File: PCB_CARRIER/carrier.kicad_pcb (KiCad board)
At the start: 6 copper layers, 69.6 x 46 mm, 87 parts, among them J1 SODIMM-260_Split, J2 Micro_SD_Card_Det2, Q1 BSS138, Q2 BSS138, Q3 BSS138, Q4 BC817-40, SW1 SW_DIP_x04, U1 SN74LVC8T245, U2 SN74LVC8T245, U3 SN74LVC8T245, U4 RT9742GGJ5

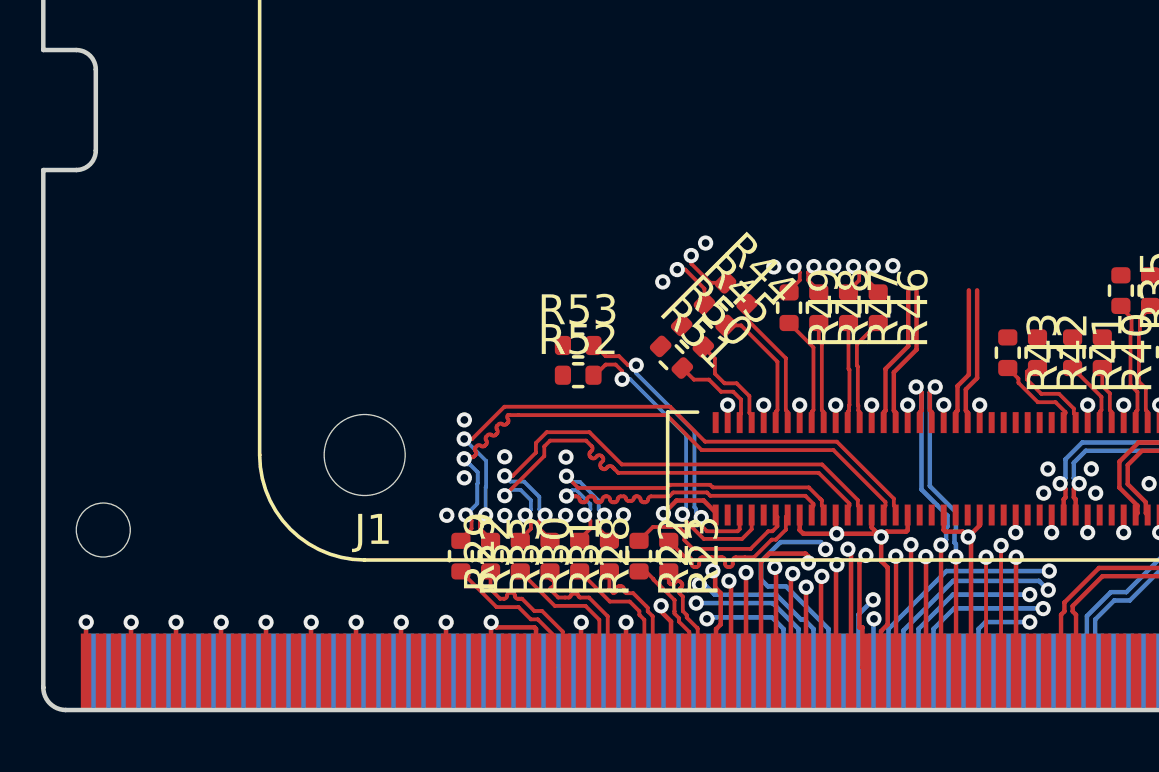
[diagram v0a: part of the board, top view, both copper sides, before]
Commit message: yes I'm still routing CSI
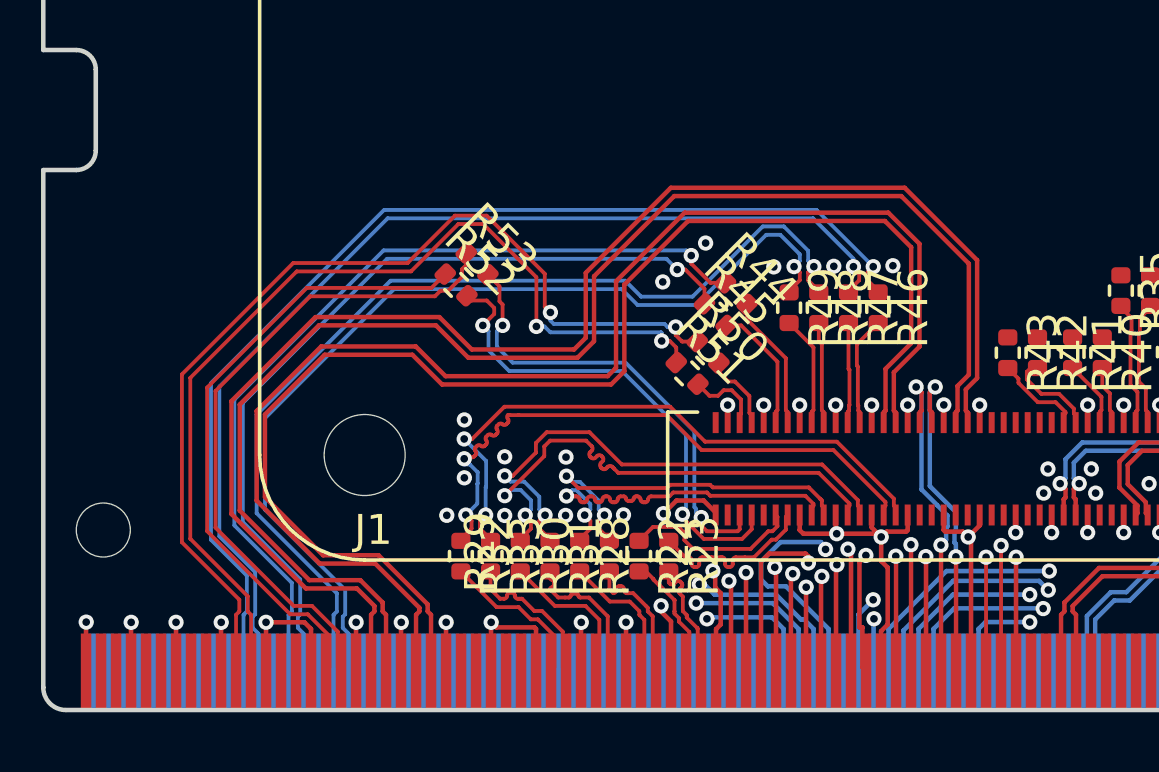
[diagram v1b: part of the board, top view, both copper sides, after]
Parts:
- moved R52 5.06 mm to (113.8, 85.8), turned to -45 degrees
- moved R53 4.33 mm to (114.5, 85.1), turned to -45 degrees
- moved R50 0.75 mm to (122.2, 88.1)
- moved R51 0.75 mm to (121.5, 88.8)
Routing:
- net USB3-1-RX_N: track 4.59 -> 48.6 mm
- net USB3-1-RX_P: track 4.59 -> 47.7 mm
- net USB3-1-TX_N: track 4.73 -> 46.2 mm
- net USB3-1-TX_P: track 4.73 -> 45.2 mm
- net dCSI-1_D0_N: track 1.08 -> 36.5 mm
- net dCSI-1_D0_P: track 1.08 -> 35.5 mm
- net dCSI-1_D2_N: track 0.00 -> 32.8 mm, vias 0 -> 2
- net dCSI-1_D2_P: track 0.00 -> 32.3 mm, vias 0 -> 2
- net dCSI-1_D1_N: track 1.09 -> 33.2 mm
- net dCSI-1_D1_P: track 1.09 -> 32.3 mm
- net dCSI-1_CLK_N: track 1.67 -> 28.9 mm
- net dCSI-1_CLK_P: track 1.67 -> 28.1 mm
- net dCSI-1_D3_P: track 0.00 -> 22.1 mm
- net dCSI-1_D3_N: track 0.00 -> 21.0 mm
- net CSI-1_D3_N: track 10.4 -> 16.5 mm
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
